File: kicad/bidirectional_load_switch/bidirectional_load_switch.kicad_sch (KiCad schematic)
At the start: 19 parts, among them J101 1017503, J102 Conn_01x02_Socket, J103 Conn_01x09_Socket, J104 Conn_01x02_Socket, U101 LDL212PV33R, U103 TMCS1101A3BQDR, U105 SN74LVC08APWR

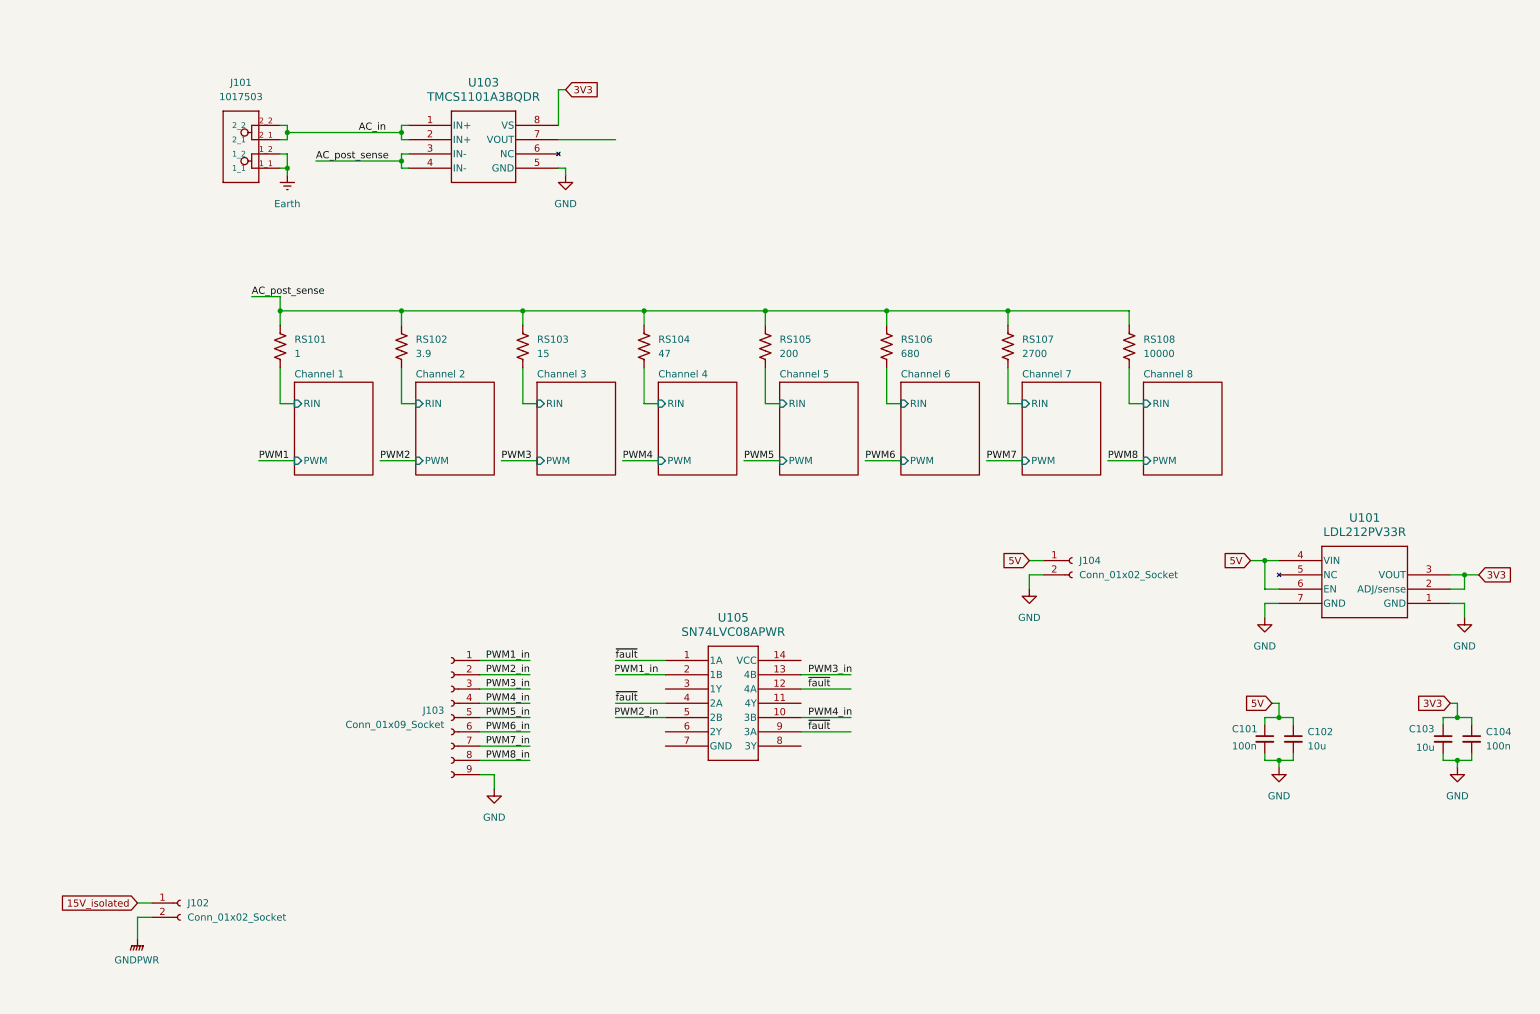
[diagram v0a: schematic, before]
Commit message: i hate layouts
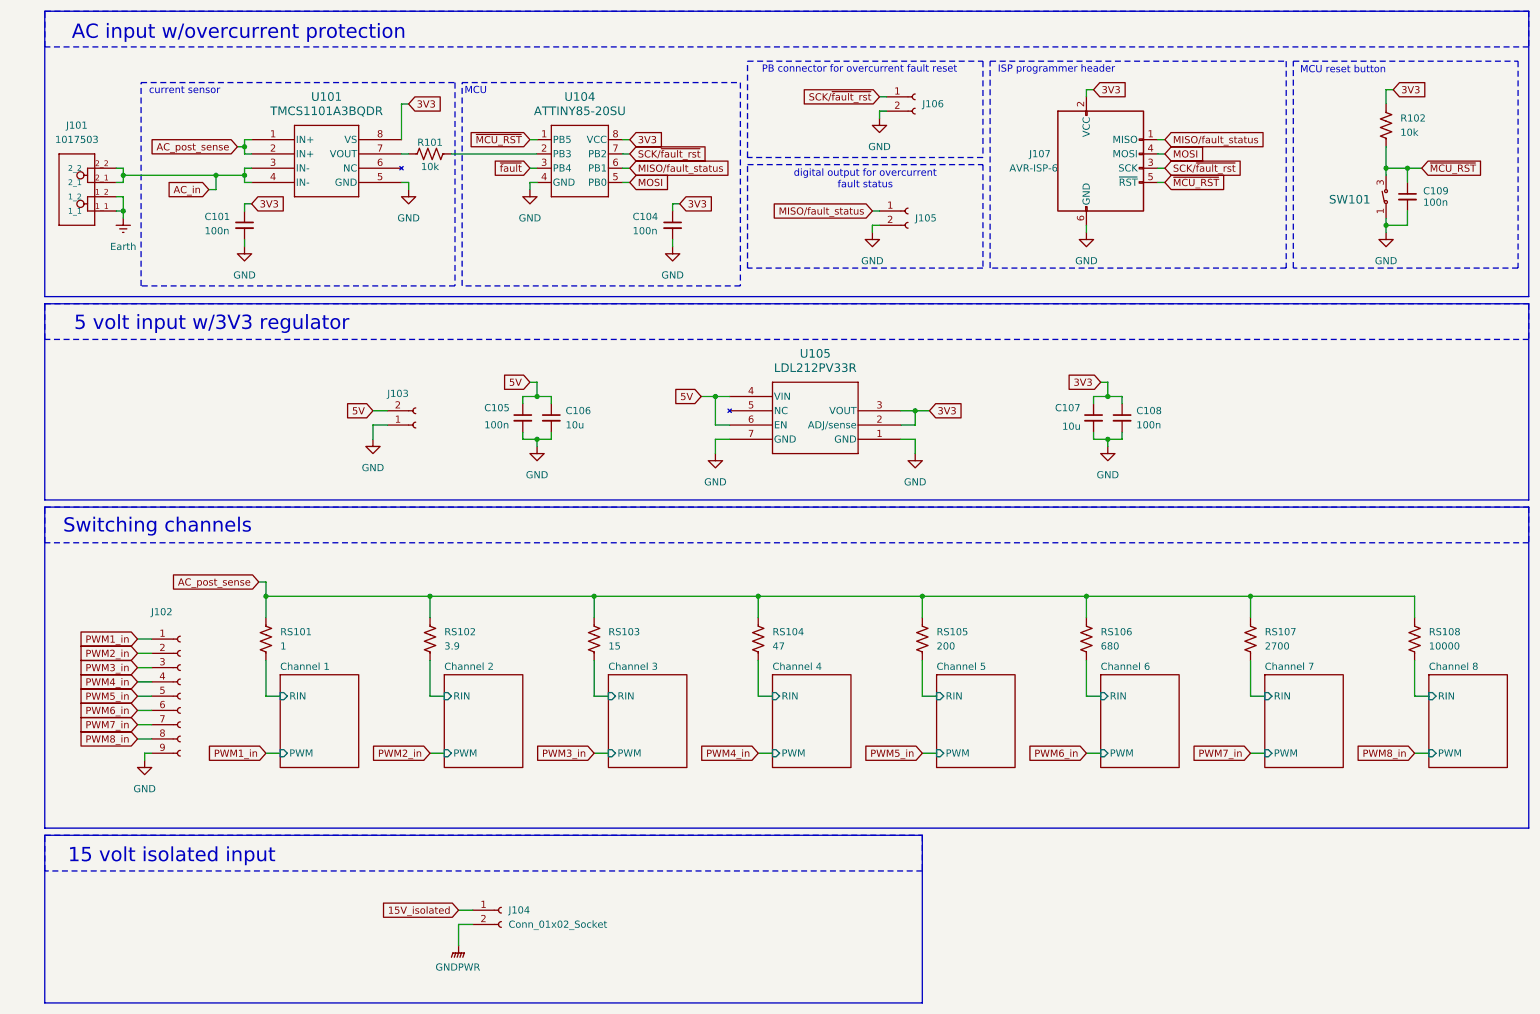
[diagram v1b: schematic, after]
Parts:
- removed U105: SN74LVC08APWR, PW14, symbol and_gate_SN74LVC08APWR:SN74LVC08APWR
- added C101, C104, C109: 100n, Capacitor_SMD:C_0603_1608Metric, symbol Device:C_Small
- added J105, J106: Conn_01x02_Socket, Connector_PinHeader_2.54mm:PinHeader_1x02_P2.54mm_Vertical, symbol Connector:Conn_01x02_Socket
- added J107: AVR-ISP-6, Connector_IDC:IDC-Header_2x03_P2.54mm_Vertical, symbol isp:AVR-ISP-6
- added R101, R102: 10k, Resistor_SMD:R_0603_1608Metric, symbol Device:R_US
- added SW101: PTS526 SK15 SMTR2 LFS, switch_switch_PTS526_SK15_SMTR2_LFS:SMT_FS, symbol switch_PTS526_SK15_SMTR2_LFS:PTS526_SK15_SMTR2_LFS
- added U104: ATTINY85-20SU, mcu_ATTINY85_20SU:8S2_ATM, symbol mcu_ATTINY85-20SU:ATTINY85-20SU
- J101: footprint 1017503:PHOENIX_1017503 -> spring_terminal_1017503:PHOENIX_1017503
- U101: renamed from U103; footprint SOIC8_D_TEX -> current_sensor_TMCS1101A3BQDR:SOIC8_D_TEX
- renumbered C101 to C105, C102 to C106, C103 to C107, C104 to C108, J103 to J102, J104 to J103, J102 to J104, U101 to U105
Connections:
- net 3V3: now also C101.1, C104.1, J107.2 (VCC), R102.1, U104.8 (VCC)
- net 5V: now also J103.2 (Pin_2); no longer J103.1 (Pin_1)
- net AC_in: now also U101.3 (IN-), U101.4 (IN-); no longer U101.1 (IN+), U101.2 (IN+)
- net AC_post_sense: now also U101.1 (IN+), U101.2 (IN+); no longer U101.3 (IN-), U101.4 (IN-)
- net GND: now also J103.1 (Pin_1), C101.2, C104.2, C109.2, J105.2 (Pin_2), J106.2 (Pin_2), J107.6 (GND), SW101.1, SW101.2, U104.4 (GND); no longer J103.2 (Pin_2)
- net ~{fault}: now also U104.3 (PB4)
- net at U101.7 (VOUT): now also R101.1
- new net: R101.2, U104.2 (PB3)
- new net MISO/fault_status: J105.1 (Pin_1), J107.1 (MISO), U104.6 (PB1)
- new net MOSI: J107.4 (MOSI), U104.5 (PB0)
- new net SCK/~{fault_rst}: J106.1 (Pin_1), J107.3 (SCK), U104.7 (PB2)
- new net ~{MCU_RST}: C109.1, J107.5 (~{RST}), R102.2, SW101.3, SW101.4, U104.1 (PB5)
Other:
- note added: "15 volt isolated input"
- note added: "5 volt input w/3V3 regulator"
- note added: "AC input w/overcurrent protection"
- note added: "ISP programmer header"
- note added: "MCU"
- note added: "MCU reset button"
- note added: "PB connector for overcurrent fault reset"
- note added: "Switching channels"
- note added: "current sensor"
- note added: "digital output for overcurrent fault status"
- moved on the sheet: C105, C106, C107, C108, J101, J102, J103, J104, RS101, RS102, RS103, RS104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
